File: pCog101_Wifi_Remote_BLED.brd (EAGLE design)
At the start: 48 x 28 mm, 59 parts, among them T1 MMBT3904LT1G, T2 PZT2907A, T3 MMBT3904LT1G, T4 MMBT3904LT1G, T5 MMBT3904LT1G, U1 PNA460XM

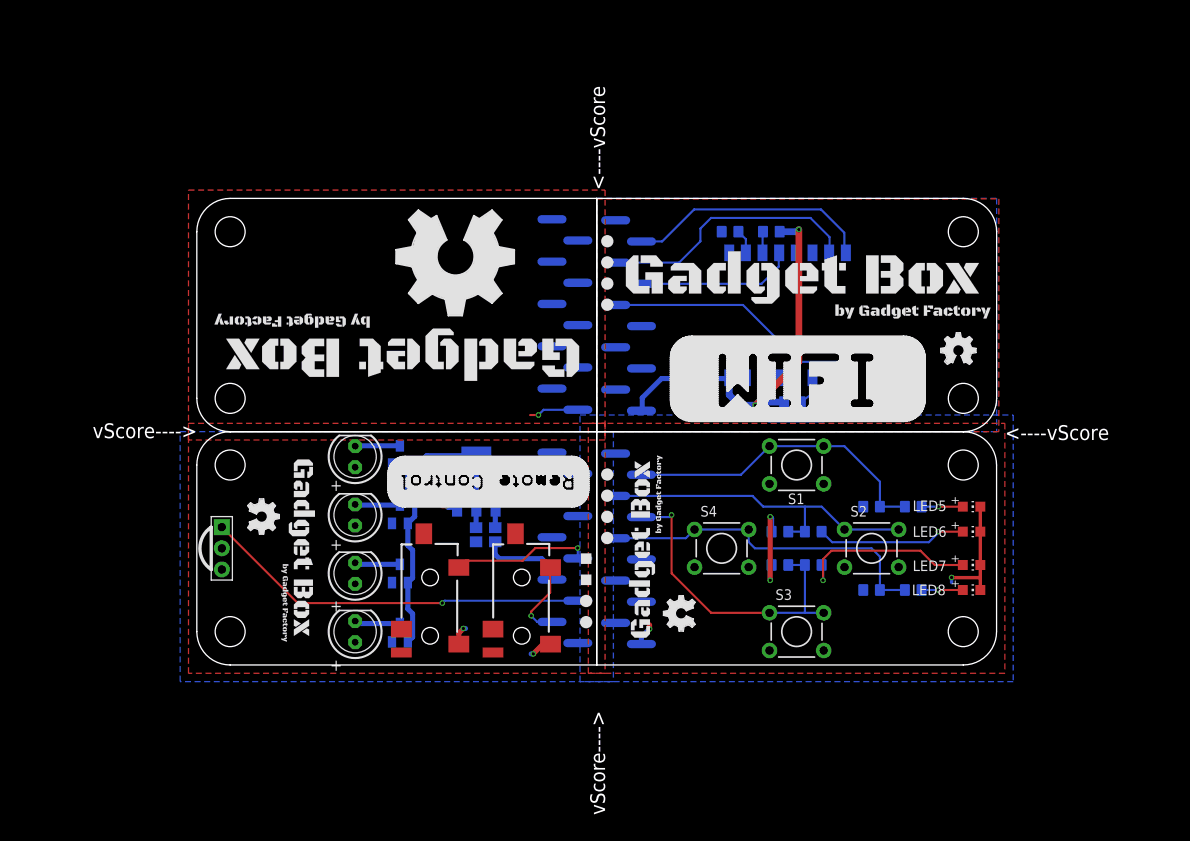
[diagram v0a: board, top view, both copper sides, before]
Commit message: All the 2.0 updates
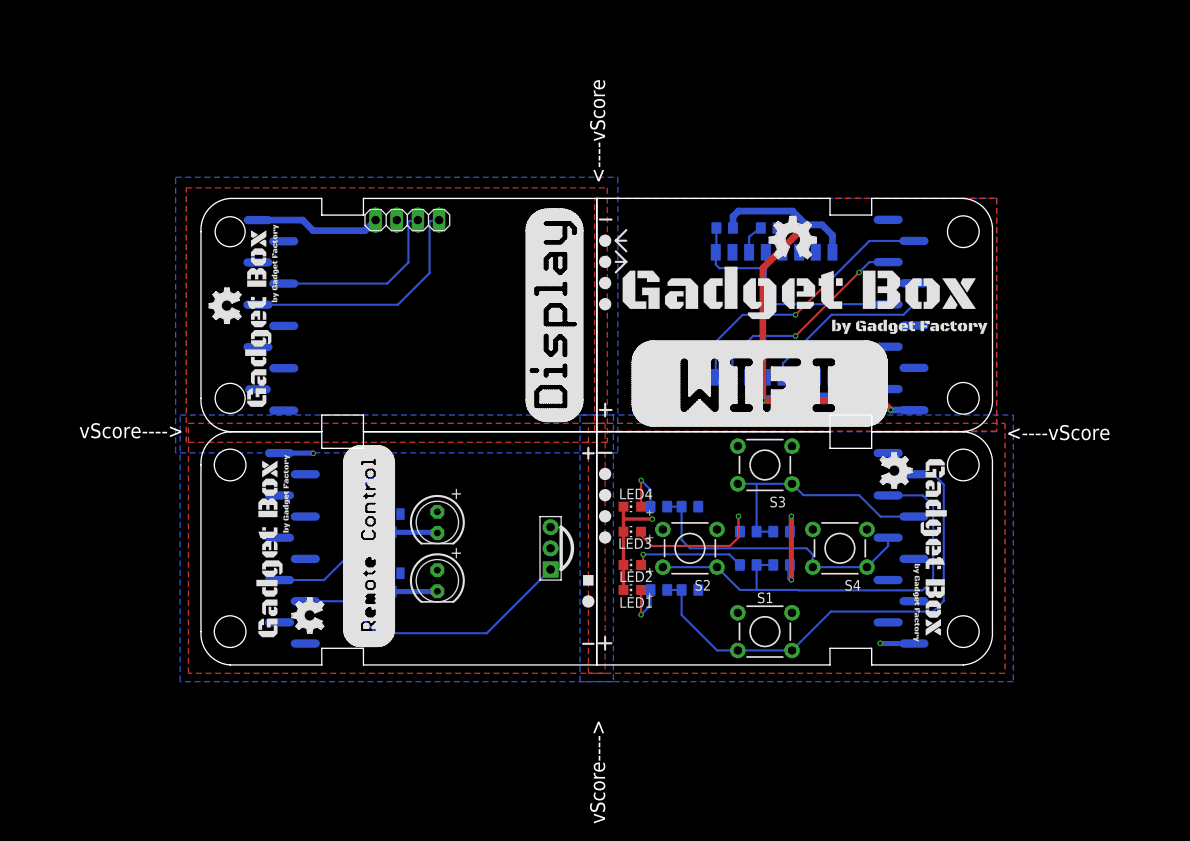
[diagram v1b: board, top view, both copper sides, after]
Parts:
- removed LED5, LED6, LED7, LED8: (no value), adafruit:CHIP-LED0805
- removed R14: 10K, GadgetFactory:0805
- removed T2: PZT2907A, zetex:SOT223
- removed T4, T5: MMBT3904LT1G, transistor:SOT23-BEC
- removed U$19: (no value), ohw-logo:OSHW_FILLX150_NOTEXT
- removed U$20: (no value), ohw-logo:OSHW_FILLX500_NOTEXT
- removed U2, U3: (no value), SparkFun:AUDIO-JACK-3.5MM-SMD
- added IR1, IR2: (no value), adafruit:LED5MM
- added JP1: .96 I2C OLED LCD, pinhead:1X04
- ECOG2: value ECOG_GENERAL_ROWECOG_GENERAL_SMD -> ECOG_BUSES_ROWECOG_BUSES_SMD; device eCogs:ECOG_GENERAL_SMD -> eCogs:ECOG_BUSES_SMD
- LED1, LED2, LED3, LED4: device adafruit:LED5MM -> adafruit:CHIP-LED0805
- R1: value 10K -> 1.0 K; device GadgetFactory:0805 -> rcl-ez:R0805
- R11, R13, R7, R9: value 390 -> 10K
- R2, R4, R8: value 10K -> 390
- R5: value 10K (opt) -> 10K; device rcl-ez:R0805 -> GadgetFactory:0805
- R6: value 1.0 K -> 390; device rcl-ez:R0805 -> GadgetFactory:0805
- U$1, U$15: device GadgetFactory:GADGETBOX_TEXT -> eCogs:LEGEND_DIO
- U$10: device GadgetFactory:GADGETBOX_SMALL -> ohw-logo:OSHW_FILLX150_NOTEXT
- U$11, U$5: device eCogs:LEGEND_DIO -> GadgetFactory:GADGETBOX_SMALL
- U$12, U$6: device eCogs:LEGEND_DIO -> ohw-logo:OSHW_FILLX150_NOTEXT
- U$13: device eCogs:LEGEND_DIO -> GadgetFactory:GADGETBOX_TEXT
- U$16: device GadgetFactory:GADGETBOX_SMALL -> eCogs:LEGEND_DIO
- U$17: device ohw-logo:OSHW_FILLX150_NOTEXT -> eCogs:LEGEND_DIO
- U$18: device ohw-logo:OSHW_FILLX150_NOTEXT -> ohw-logo:OSHW_FILLX200_NOTEXT
- U$2: device eCogs:LEGEND_DIO -> eCogs:LEGEND_PWM
- U$8: device eCogs:LEGEND_PWM -> eCogs:LEGEND_DIO
- U$9: device eCogs:LEGEND_PWM -> GadgetFactory:GADGETBOX_SMALL
- moved U$10 70.4 mm to (82.0, 25.5)
- moved ECOG 55.6 mm to (0.00, 0.00)
- moved ECOG2 55.6 mm to (-0.00, 28.0)
- moved R1 55.4 mm to (22.6, 21.5), turned to 270 degrees
- moved U$17 52.9 mm to (49.0, 50.9), turned to 180 degrees
- moved U$5 49.9 mm to (8.79, 14.0), turned to 90 degrees
- moved U$12 48.6 mm to (5.30, 41.0), turned to 90 degrees
- moved ECOG3 48.0 mm to (96.0, 56.0)
- moved ECOG1 48.0 mm to (96.0, 28.0)
- moved R13 46.8 mm to (68.7, 52.4)
- moved U$11 45.8 mm to (7.45, 41.6), turned to 90 degrees
- moved U$18 45.6 mm to (68.7, 48.8), turned to 0 degrees
- moved R2 43.8 mm to (55.5, 9.00), turned to 0 degrees
- moved U$9 41.7 mm to (88.4, 14.0), turned to 270 degrees
- moved R12 41.0 mm to (63.4, 52.4)
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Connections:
- removed net N$13: LED8.A, R13.2
- removed net RX: ECOG.G1, X1.15
- removed net TX: ECOG.G0, X1.16
- new net RX/MOSI: ECOG3.G1, X1.15
- new net TX/MISO: ECOG3.G0, X1.16
- net 1: now also ECOG1.G0, R2.1, R3.2; no longer ECOG2.G0, R7.1, R8.2
- net 2: now also ECOG1.G1, R4.1, R5.2; no longer ECOG2.G1, R10.2, R9.1
- net 3: now also ECOG1.G2, R6.1, R7.2; no longer ECOG2.G2, R11.1, R12.2
- net 3V3: now also IR1.A, IR2.A, JP1.1, R10.2, R12.2, R13.2; no longer LED1.A, LED2.A, LED3.A, LED4.A, R1.2, R3.2, R4.2, T2.3, U2.RING
- net 4: now also ECOG1.G3, R8.1, R9.2; no longer ECOG2.G3, R13.1, R14.2
- net BLAST_RX: now also ECOG.G0; no longer ECOG1.G0, U2.TIP
- net BLAST_TX: now also ECOG.G3; no longer ECOG1.G3, U3.TIP
- net GND: now also JP1.2, LED1.C, LED2.C, LED3.C, LED4.C, R11.1, R3.1, R7.1, R9.1; no longer LED5.C, LED6.C, LED7.C, LED8.C, R10.1, R12.1, R14.1, R2.1, R8.1, T4.E, T5.E, U2.SLEEVE, U3.SLEEVE
- net GPIO0/BOOTLOAD: now also ECOG3.G2; no longer ECOG.G2
- net N$1: now also LED1.A, R2.2; no longer LED5.A, R7.2
- net N$10: now also R1.2; no longer R5.2, T2.2, T2.4, T4.B, T5.B
- net N$11: now also R11.2, X1.10; no longer LED4.K, T5.C
- net N$12: now also R13.1, X1.3; no longer LED7.A, R11.2
- net N$2: now also LED2.A, R4.2; no longer LED6.A, R9.2
- net N$3: now also LED3.A, R6.2; no longer R1.1, X1.11
- net N$4: now also LED4.A, R8.2; no longer R2.2, X1.10
- net N$5: now also ECOG2.I2C-SDA, JP1.4; no longer R4.1, X1.3
- net N$6: now also ECOG2.I2C-SCL, JP1.3; no longer R6.1, T2.1
- net N$7: now also IR1.K; no longer LED1.K
- net N$8: now also R10.1, X1.11; no longer LED3.K, T4.C
- net N$9: now also IR2.K; no longer LED2.K
- net RECEIVE: now also ECOG.G1; no longer ECOG1.G1
- net RESET: now also ECOG3.G3, R12.1; no longer ECOG.G3, R3.1
- net TRANSMIT: now also ECOG.G2, R1.1; no longer ECOG1.G2, R6.2
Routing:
- net TX/MISO: track 0.00 -> 33.3 mm, vias 0 -> 2
- net RX: track 31.6 -> 0.00 mm
- net N$10: track 40.3 -> 9.72 mm
- net TX: track 29.6 -> 0.00 mm
- net N$5: track 3.63 -> 29.5 mm
- net RX/MOSI: track 0.00 -> 25.9 mm, vias 0 -> 2
- net 3V3: track 65.7 -> 88.1 mm
- net 1: track 37.8 -> 58.5 mm
- net N$6: track 2.46 -> 22.1 mm
- net N$12: track 22.4 -> 3.63 mm, vias 1 -> 0
- net BLAST_TX: track 16.5 -> 0.00 mm, vias 1 -> 0
- net N$3: track 2.56 -> 18.2 mm, vias 0 -> 1
- net 2: track 40.6 -> 53.9 mm
- net RECEIVE: track 46.6 -> 34.2 mm, vias 1 -> 0
- net GND: track 36.6 -> 24.8 mm, vias 6 -> 3
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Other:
- board size 48 x 28 mm -> 47.5 x 28 mm
- board text added: "0"
- board text added: "1"
- board text added: "2"
- board text added: "3"
- board text added: "I2C-SCL"
- board text added: "I2C-SDA"
- board text added: "L/S1"
- board text added: "L/S2"
- board text added: "L/S3"
- board text added: "L/S4"
- board text added: "OLED LCD I2C"
- board text added: "RECEIVE"
- board text added: "RX/MOSI"
- board text added: "TRANSMIT"
- board text added: "TX/MISO"
- board text added: "ecog100 v2.0"
- board text added: "ecog101 v2.0"
- board text added: "ecog101.GadgetFactory.net"
- board text added: "ecog106 v2.0"
- board text added: "ecog107 v2.0"
- board text removed: "BLAST_RX<"
- board text removed: "BLAST_TX>"
- board text removed: "Blank"
- board text removed: "P1<>"
- board text removed: "P2<>"
- board text removed: "P3<>"
- board text removed: "P4<>"
- board text removed: "RECEIVE<"
- board text removed: "RX>"
- board text removed: "TRANSMIT>"
- board text removed: "TX<"
- board text removed: "ecog0 v1.4"
- board text removed: "ecog0.GadgetFactory.net"
- board text removed: "ecog100 v1.1"
- board text removed: "ecog106 v1.1"
- board text removed: "ecog107 v1.0"
